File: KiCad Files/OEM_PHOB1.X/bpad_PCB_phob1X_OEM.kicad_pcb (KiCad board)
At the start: 2 copper layers, 31.6 x 51.6 mm, 28 parts, among them J1 Conn_01x04, SW1 C_left, SW2 C_up, SW3 C_down, SW4 C_right

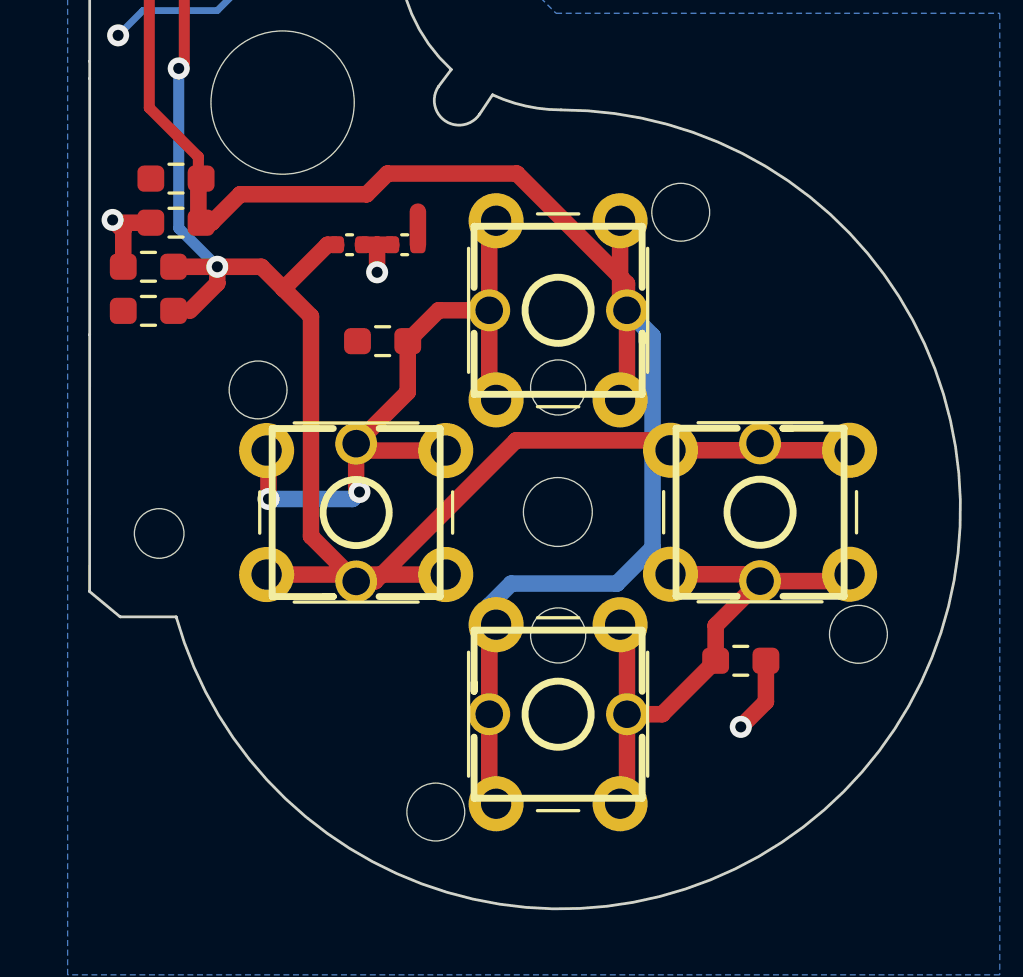
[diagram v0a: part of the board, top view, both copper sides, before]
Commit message: cleaned up and fixed
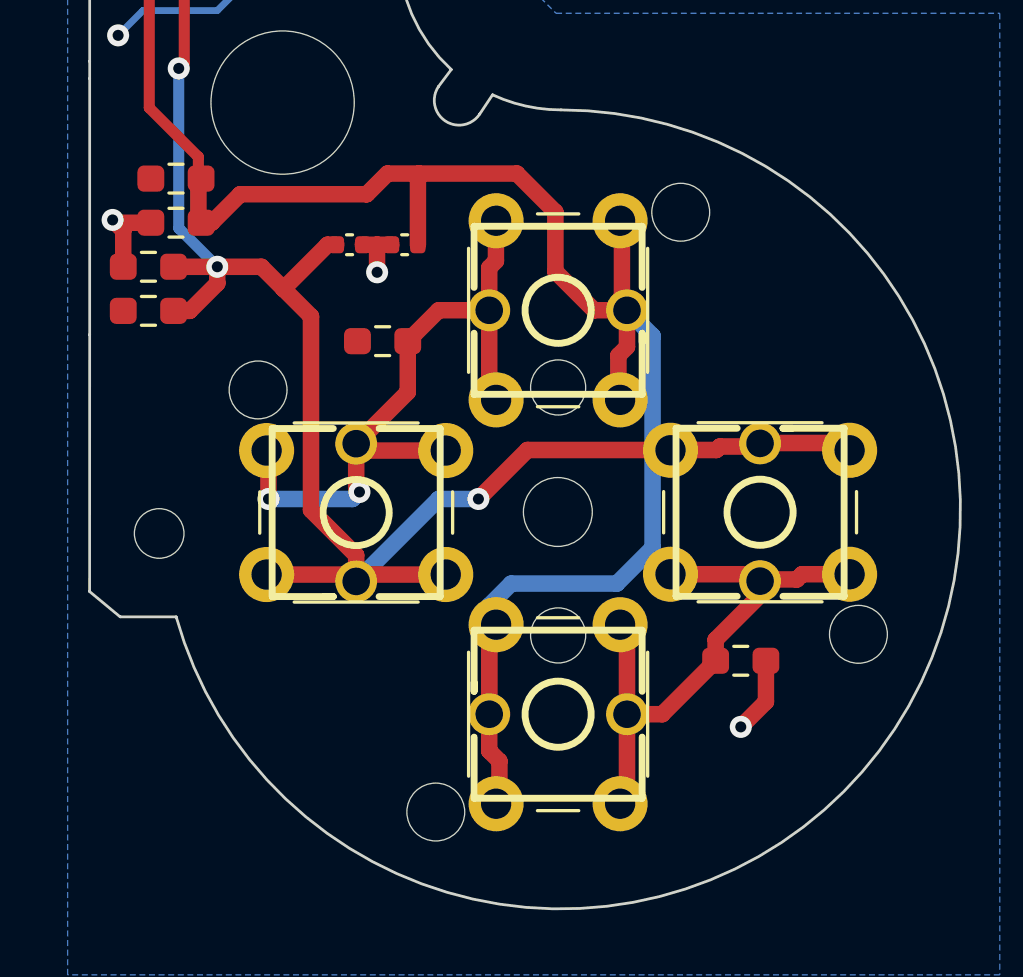
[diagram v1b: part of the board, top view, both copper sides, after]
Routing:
- net /C_x: track 80.5 -> 83.1 mm
- net /C_y: track 73.9 -> 73.6 mm, vias 2 -> 3
